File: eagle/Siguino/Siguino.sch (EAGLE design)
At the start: 34 parts, among them J1 FTDI Basic, Q1 MOSFET P-CH 20V 5.3A SOT-23, U1 ATMEGA328P_TQFP, U2 AT30TS750ATSSOP, U3 LIS3DH, Y1 8MHz

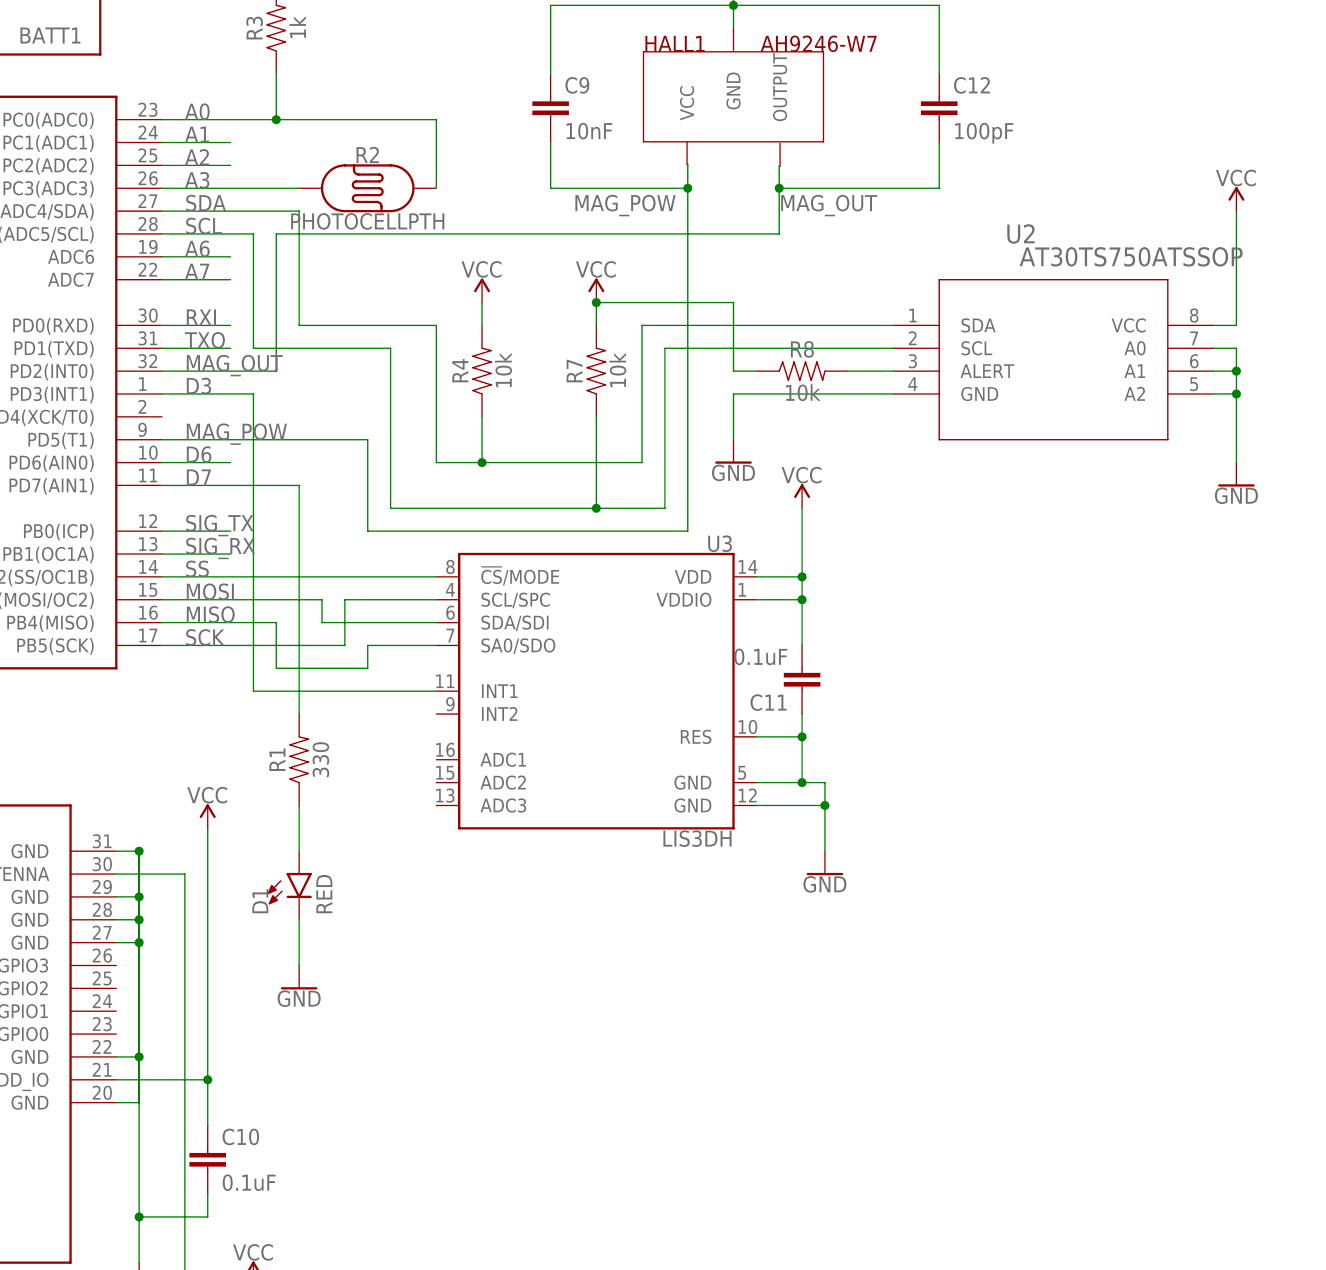
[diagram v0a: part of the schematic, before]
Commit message: Updated with latest 0.5 and 1.0 changes
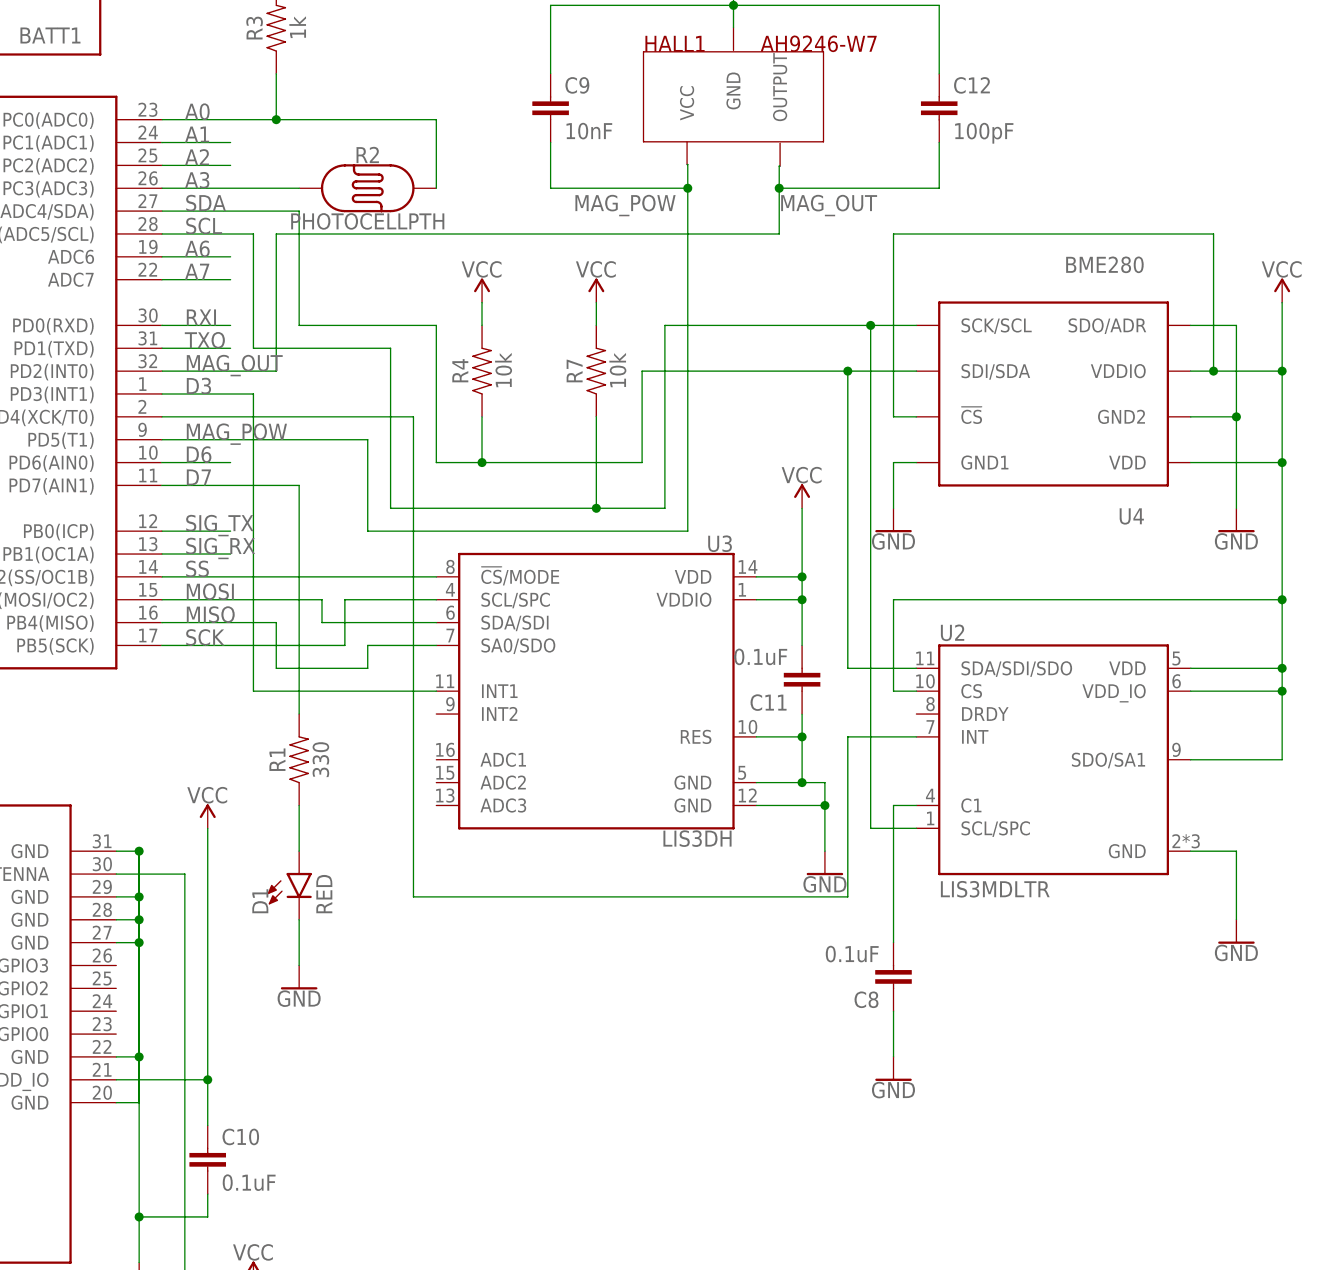
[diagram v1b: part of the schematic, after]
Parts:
- removed R8: 10k, SparkFun-Resistors:10KOHM-0603-1/10W-1%
- added C8: 0.1uF, SparkFun-Capacitors:0.1UF-0603-25V-5%
- added U4: BME280, BME280ComponentLibrary:BME280
- U2: value AT30TS750ATSSOP -> LIS3MDLTR; device DigiKey:AT30TS750ATSSOP -> LIS3MDLTR:LIS3MDLTR
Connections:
- removed net N$8: R8.2, U2.ALERT
- new net N$11: U1.PD4(XCK/T0), U2.INT
- new net N$9: C8.2, U2.C1
- net GND: now also C8.1, U4.GND1, U4.GND2, U4.SDO/ADR; no longer U2.A0, U2.A1, U2.A2
- net SCL: now also U2.SCL/SPC, U4.SCK/SCL; no longer U2.SCL
- net SDA: now also U2.SDA/SDI/SDO, U4.SDI/SDA; no longer U2.SDA
- net VCC: now also U2.CS, U2.SDO/SA1, U2.VDD, U2.VDD_IO, U4.!CS, U4.VDD, U4.VDDIO; no longer R8.1, U2.VCC

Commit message: Cleaned schematic & changed antenna path on Board
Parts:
- ANT1: device proant:PRO-OB-512ONBOARD -> Siguino:PROANT_PRO-OB-512ONBOARD
- BATT1: value CR2-BATTERY-HOLDERPTH -> SPARKFUN-BATTERIES_CR2-BATTERY-HOLDERPTH; device SparkFun-Batteries:CR2-BATTERY-HOLDERPTH -> Siguino:SPARKFUN-BATTERIES_CR2-BATTERY-HOLDERPTH
- C8: value 0.1uF -> 100nF
- HALL1: value AH9246-W7 -> TR-J_AH9246-W7; device tr-j:AH9246-W7 -> Siguino:TR-J_AH9246-W7
- SFM1: device WiSOL:WSSFM10'HANDSOLDER' -> Siguino:WISOL_WSSFM10HANDSOLDER
- U2: value LIS3MDLTR -> LIS3MDLTR_LIS3MDLTR; device LIS3MDLTR:LIS3MDLTR -> Siguino:LIS3MDLTR_LIS3MDLTR
- U3: value LIS3DH -> SPARKFUN-SENSORS_LIS3DH; device SparkFun-Sensors:LIS3DH -> Siguino:SPARKFUN-SENSORS_LIS3DH
- U4: device BME280ComponentLibrary:BME280 -> Siguino:BME280COMPONENTLIBRARY_BME280
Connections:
- net A0 renamed LIGHT_SENSE
- net A3 renamed LIGHT_POWER
- net D3 renamed INT1
- net MAG_OUT renamed HALL_SENSE
- net MAG_POW renamed HALL_POWER
- net N$11 renamed MAG_INT
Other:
- note added: "Accellerometer Sensor"
- note added: "Hall Sensor"
- note added: "Header J2"
- note added: "Header J3"
- note added: "I2C Pullups"
- note added: "LED"
- note added: "Light Sensor"
- note added: "MCU Reset circuit"
- note added: "Magnetometer Sensor"
- note added: "Microcontroller"
- note added: "Power supply"
- note added: "Programmer"
- note added: "Sigfox Radio module"
- note added: "Temperature & Humidity Sensor"
- moved on the sheet: C1, C10, C11, C12, C13, C15, C2, C3, C4, C5, C6, C7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
